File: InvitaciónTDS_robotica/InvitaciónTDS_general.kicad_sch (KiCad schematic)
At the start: 17 parts, among them J1 Voltage Conn, J2 FTDI Connector, Q7 2N2219, SW1 SW_Push, U1 LM358, U2 74LS08

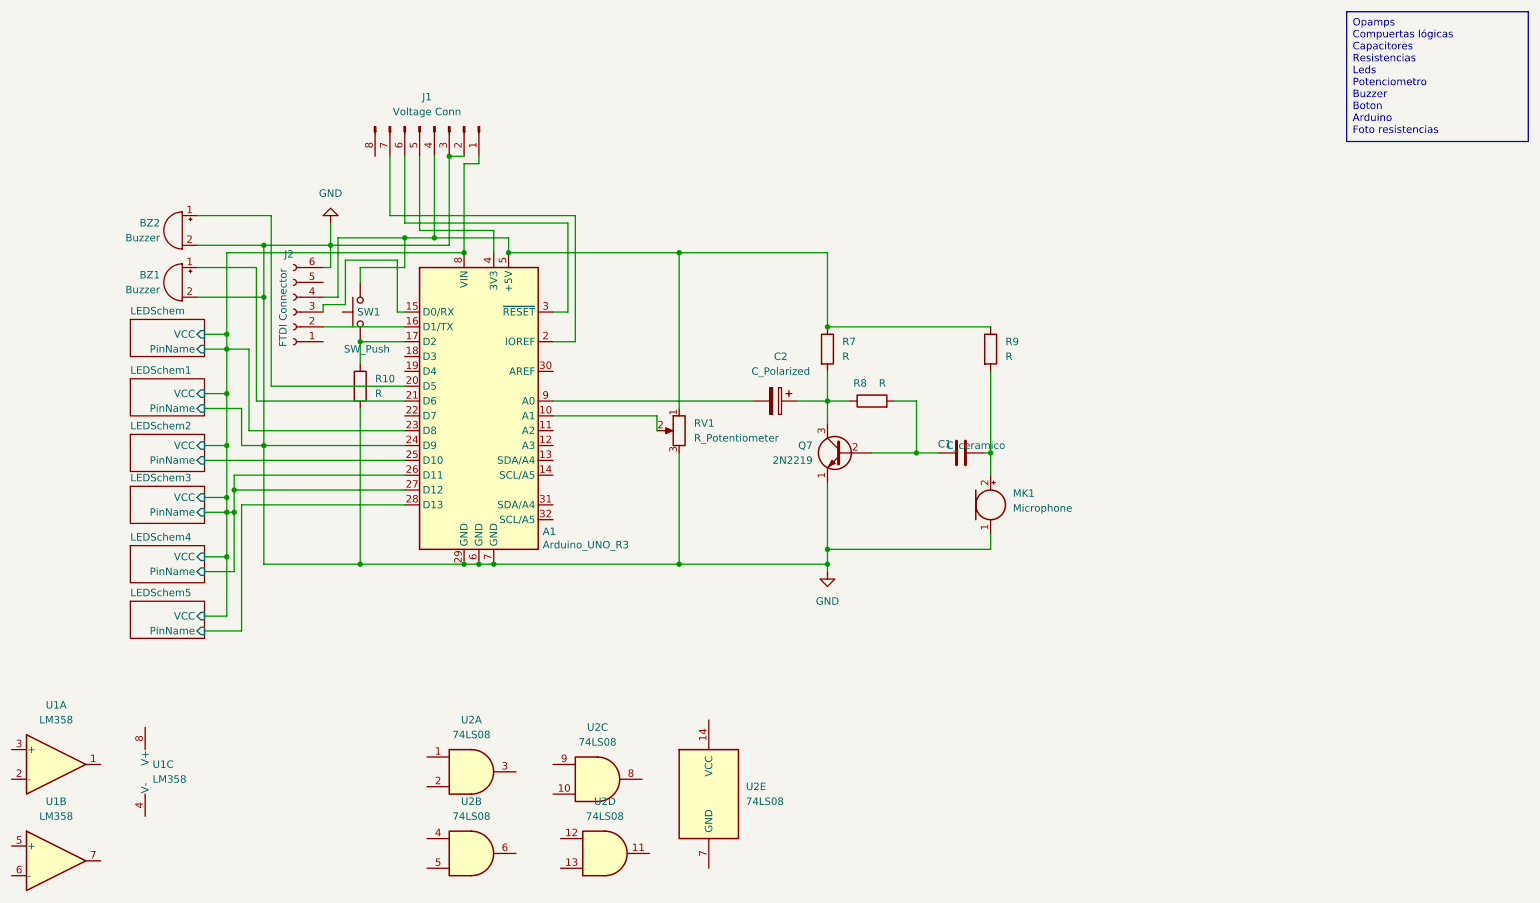
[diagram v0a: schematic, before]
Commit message: update robotica
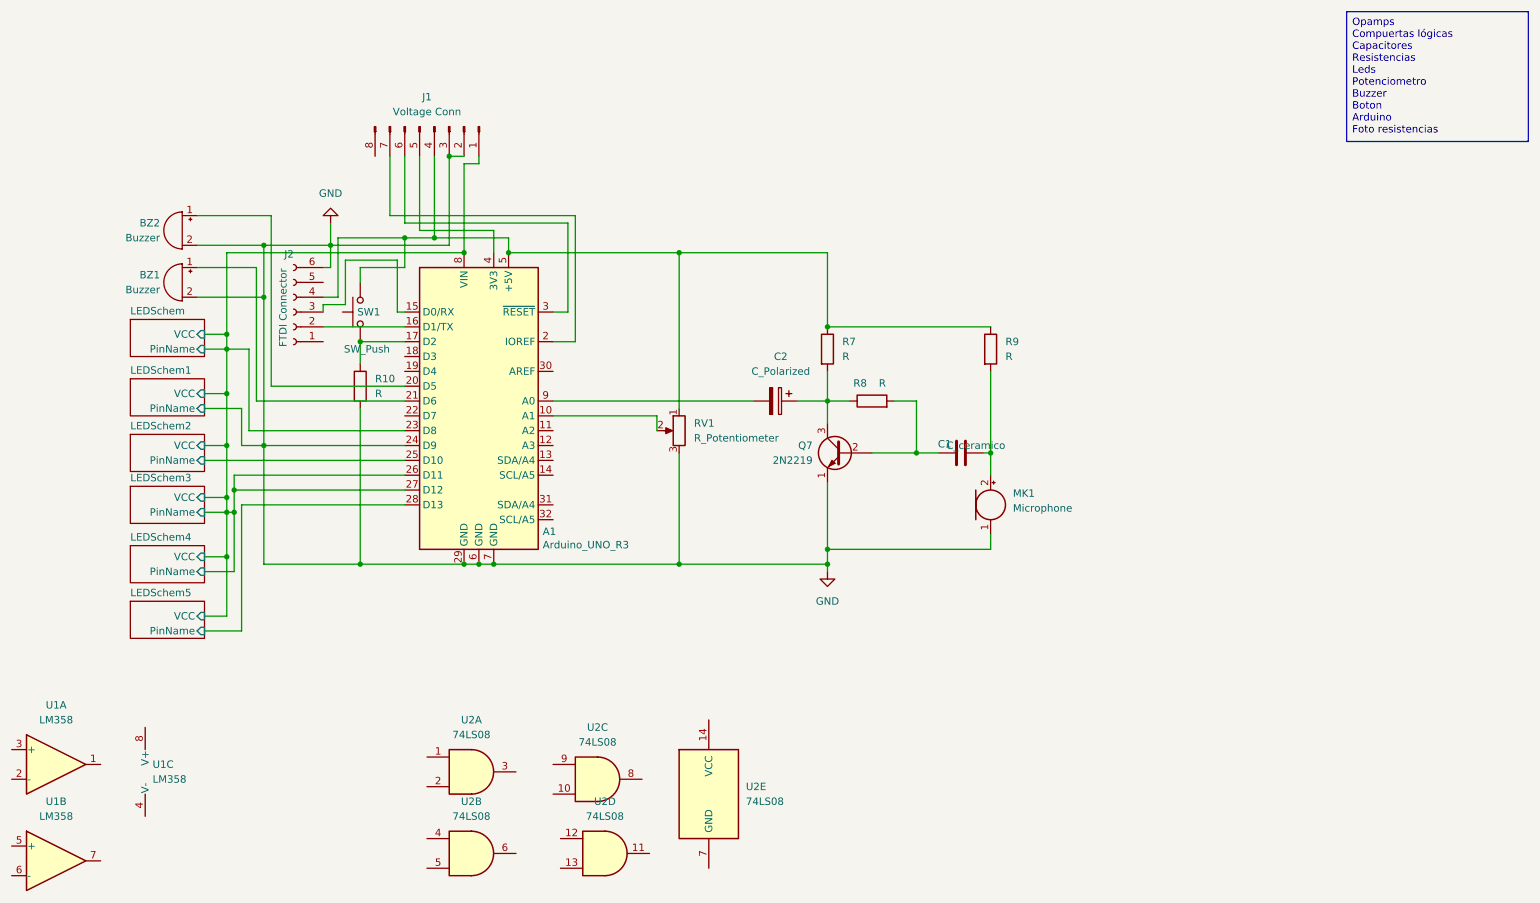
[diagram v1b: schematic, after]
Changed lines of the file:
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@@
 (kicad_sch
-	(version 20231120)
+	(version 20250114)
 	(generator "eeschema")
-	(generator_version "8.0")
+	(generator_version "9.0")
 	(paper "A4")
+	(text_box "Opamps\nCompuertas lógicas\nCapacitores\nResistencias\nLeds\nPotenciometro\nBuzzer\nBoton\nArduino\nFoto resistencias\n"
+		(exclude_from_sim no)
+		(at 251.46 42.545 0)
+		(size 31.115 22.225)
+		(margins 0.9525 0.9525 0.9525 0.9525)
+		(stroke
+			(width 0)
+			(type default)
+		)
+		(fill
+			(type none)
+		)
+		(effects
+			(font
+				(size 1.27 1.27)
+			)
+			(justify left top)
+		)
+	)
 	(junction
 		(at 59.69 128.27)
@@
 			"9QBk43qALbV69VW1GjbMsl2hQiQAAAAAAADc3uxt3QEAAAAAAACUfIRIAAAAAAAAsESIBAAAAAAA"
 			"AEuESAAAAAAAALBEiAQAAAAAAABLhEgAAAAAAACwRIgEAAAAAAAAS4RIAAAAAAAAsESIBAAAAAAA"
-			"AEv/D98C9Ad616Q4AAAAAElFTkSuQmCC"
-		)
-	)
-	(text_box "Opamps\nCompuertas lógicas\nCapacitores\nResistencias\nLeds\nPotenciometro\nBuzzer\nBoton\nArduino\nFoto resistencias\n"
-		(exclude_from_sim no)
-		(at 251.46 42.545 0)
-		(size 31.115 22.225)
-		(stroke
-			(width 0)
-			(type default)
-		)
-		(fill
-			(type none)
-		)
-		(effects
-			(font
-				(size 1.27 1.27)
-			)
-			(justify left top)
+			"AEv/D98C9Ad616Q4AAAAAElFTkSuQmCCAAAAAAAAAAAAAAAAAAAAAAAAAAAAAAAAAAAAAAAAAAAA"
+			"AAAAAAAAAAAAAAAAAAAAAAAAAAAAAAAAAAAAAAAAAAAAAAAAAAAAAAAAAAAAAAAAAAAAAAAAAAAA"
+			"AAAAAAAAAAAAAAAAAAAAAAAAAAAAAAAAAAAAAAAAAAAAAAAAAAAAAAAAAAAAAAAAAAAAAAAAAAAA"
+			"AAAAAAAAAAAAAAAAAAAAAAAAAAAAAAAAAAAAAAAAAAAAAAAAAAAAAAAAAAAAAAAAAAAAAAAAAAAA"
+			"AAAAAAAAAAAAAAAAAAAAAAAAAAAAAAAAAAAAAAAAAAAAAAAAAAAAAAAAAAAAAAAAAAAAAAAAAAAA"
+			"AAAAAAAAAAAAAAAAAAAAAAAAAAAAAAAAAAAAAAAAAAAAAAAAAAAAAAAAAAAAAAAAAAAAAAAAAAAA"
+			"AAAAAAAAAAAAAAAAAAAAAAAAAAAAAAAAAAAAAAAAAAAAAAAAAAAAAAAAAAAAAAAAAAAAAAAAAAAA"
+			"AAAAAAAAAAAAAAAAAAAAAAAAAAAAAAAAAAAAAAAAAAAAAAAAAAAAAAAAAAAAAAAAAAAAAAAAAAAA"
+			"AAAAAAAAAAAAAAAAAAAAAAAAAAAAAAAAAAAAAAAAAAAAAAAAAAAAAAAAAAAAAAAAAAAAAAAAAAAA"
+			"AAAAAAAAAAAAAAAAAAAAAAAAAAAAAAAAAAAAAAAAAAAAAAAAAAAAAAAAAAAAAAAAAAAAAAAAAAAA"
+			"AAAAAAAAAAAAAAAAAAAAAAAAAAAAAAAAAAAAAAAAAAAAAAAAAAAAAAAAAAAAAAAAAAAAAAAAAAAA"
+			"AAAAAAAAAAAAAAAAAAAAAAAAAAAAAAAAAAAAAAAAAAAAAAAAAAAAAAAAAAAAAAAAAAAAAAAAAAAA"
+			"AAAAAAAAAAAAAAAAAAAAAAAAAAAAAAAAAAAAAAAAAAAAAAAAAAAAAAAAAAAAAAAAAAAAAAAAAAAA"
+			"AAAAAAAAAAAAAAAAAAAAAAAAAAAAAAAAAAAAAAAAAAAAAAAAAAAAAAAAAAAAAAAAAAAAAAAAAAAA"
+			"AAAAAAAAAAAAAAAAAAAAAAAAAAAAAAAAAAAAAAAAAAAAAAAAAAAAAAAAAAAAAAAAAAAAAAAAAAAA"
+			"AAAAAAAAAAAAAAAAAAAAAAAAAAAAAAAAAAAAAAAAAAAAAAAAAAAAAAAAAAAAAAAAAAAAAAAAAAAA"
+			"AAAAAAAAAAAAAAAAAAAAAAAAAAAAAAAAAAAAAAAAAAAAAAAAAAAAAAAAAAAAAAAAAAAAAAAAAAAA"
+			"AAAAAAAAAAAAAAAAAAAAAAAAAAAAAAAAAAAAAAAAAAAAAAAAAAAAAAAAAAAAAAAAAAAAAAAAAAAA"
+			"AAAAAAAAAAAAAAAAAAAAAAAAAAAAAA=="
 		)
 	)
@@
 		(at 43.18 95.25)
 		(size 12.7 6.35)
+		(exclude_from_sim no)
+		(in_bom yes)
+		(on_board yes)
+		(dnp no)
 		(stroke
 			(width 0.1524)
@@
 		(at 43.18 123.825)
 		(size 12.7 6.35)
+		(exclude_from_sim no)
+		(in_bom yes)
+		(on_board yes)
+		(dnp no)
 		(stroke
 			(width 0.1524)
@@
 		(at 43.18 143.51)
 		(size 12.7 6.35)
+		(exclude_from_sim no)
+		(in_bom yes)
+		(on_board yes)
+		(dnp no)
 		(stroke
 			(width 0.1524)
@@
 		(at 43.18 133.985)
 		(size 12.7 6.35)
+		(exclude_from_sim no)
+		(in_bom yes)
+		(on_board yes)
+		(dnp no)
 		(stroke
 			(width 0.1524)
@@
 		(at 43.18 114.935)
 		(size 12.7 6.35)
+		(exclude_from_sim no)
+		(in_bom yes)
+		(on_board yes)
+		(dnp no)
 		(stroke
 			(width 0.1524)
@@
 		(at 43.18 105.41)
 		(size 12.7 6.35)
+		(exclude_from_sim no)
+		(in_bom yes)
+		(on_board yes)
+		(dnp no)
 		(stroke
 			(width 0.1524)
@@
 		)
 	)
+	(embedded_fonts no)
 )

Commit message: terminado
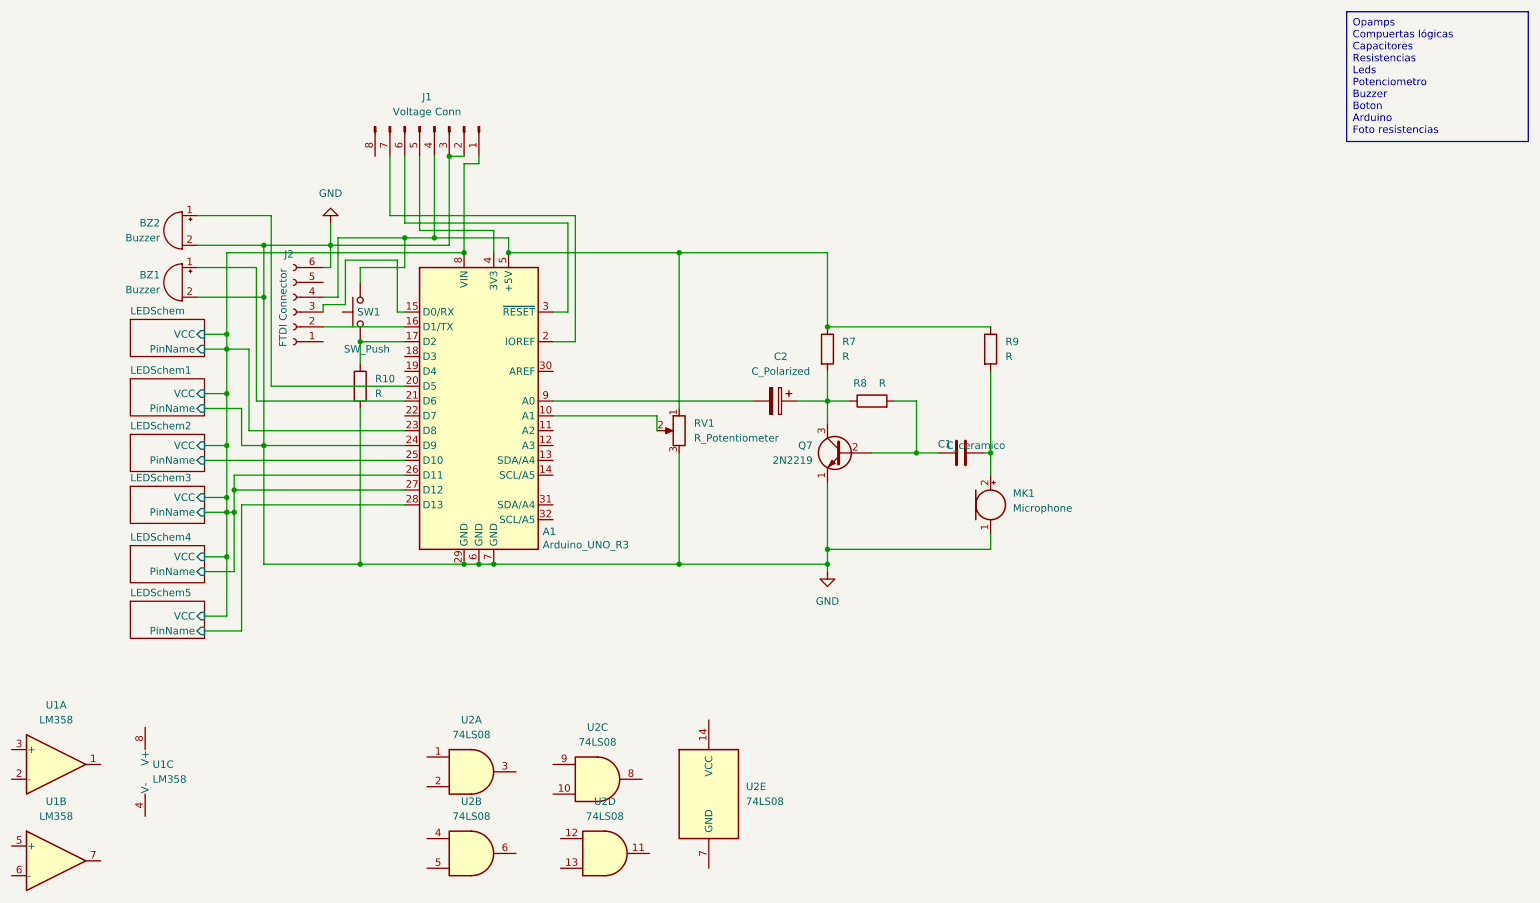
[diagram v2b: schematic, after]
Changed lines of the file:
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@@
 (kicad_sch
-	(version 20250114)
+	(version 20231120)
 	(generator "eeschema")
-	(generator_version "9.0")
+	(generator_version "8.0")
 	(paper "A4")
-	(text_box "Opamps\nCompuertas lógicas\nCapacitores\nResistencias\nLeds\nPotenciometro\nBuzzer\nBoton\nArduino\nFoto resistencias\n"
-		(exclude_from_sim no)
-		(at 251.46 42.545 0)
-		(size 31.115 22.225)
-		(margins 0.9525 0.9525 0.9525 0.9525)
-		(stroke
-			(width 0)
-			(type default)
-		)
-		(fill
-			(type none)
-		)
-		(effects
-			(font
-				(size 1.27 1.27)
-			)
-			(justify left top)
-		)
-	)
 	(junction
 		(at 59.69 128.27)
@@
 			"9QBk43qALbV69VW1GjbMsl2hQiQAAAAAAADc3uxt3QEAAAAAAACUfIRIAAAAAAAAsESIBAAAAAAA"
 			"AEuESAAAAAAAALBEiAQAAAAAAABLhEgAAAAAAACwRIgEAAAAAAAAS4RIAAAAAAAAsESIBAAAAAAA"
-			"AEv/D98C9Ad616Q4AAAAAElFTkSuQmCCAAAAAAAAAAAAAAAAAAAAAAAAAAAAAAAAAAAAAAAAAAAA"
-			"AAAAAAAAAAAAAAAAAAAAAAAAAAAAAAAAAAAAAAAAAAAAAAAAAAAAAAAAAAAAAAAAAAAAAAAAAAAA"
-			"AAAAAAAAAAAAAAAAAAAAAAAAAAAAAAAAAAAAAAAAAAAAAAAAAAAAAAAAAAAAAAAAAAAAAAAAAAAA"
-			"AAAAAAAAAAAAAAAAAAAAAAAAAAAAAAAAAAAAAAAAAAAAAAAAAAAAAAAAAAAAAAAAAAAAAAAAAAAA"
-			"AAAAAAAAAAAAAAAAAAAAAAAAAAAAAAAAAAAAAAAAAAAAAAAAAAAAAAAAAAAAAAAAAAAAAAAAAAAA"
-			"AAAAAAAAAAAAAAAAAAAAAAAAAAAAAAAAAAAAAAAAAAAAAAAAAAAAAAAAAAAAAAAAAAAAAAAAAAAA"
-			"AAAAAAAAAAAAAAAAAAAAAAAAAAAAAAAAAAAAAAAAAAAAAAAAAAAAAAAAAAAAAAAAAAAAAAAAAAAA"
-			"AAAAAAAAAAAAAAAAAAAAAAAAAAAAAAAAAAAAAAAAAAAAAAAAAAAAAAAAAAAAAAAAAAAAAAAAAAAA"
-			"AAAAAAAAAAAAAAAAAAAAAAAAAAAAAAAAAAAAAAAAAAAAAAAAAAAAAAAAAAAAAAAAAAAAAAAAAAAA"
-			"AAAAAAAAAAAAAAAAAAAAAAAAAAAAAAAAAAAAAAAAAAAAAAAAAAAAAAAAAAAAAAAAAAAAAAAAAAAA"
-			"AAAAAAAAAAAAAAAAAAAAAAAAAAAAAAAAAAAAAAAAAAAAAAAAAAAAAAAAAAAAAAAAAAAAAAAAAAAA"
-			"AAAAAAAAAAAAAAAAAAAAAAAAAAAAAAAAAAAAAAAAAAAAAAAAAAAAAAAAAAAAAAAAAAAAAAAAAAAA"
-			"AAAAAAAAAAAAAAAAAAAAAAAAAAAAAAAAAAAAAAAAAAAAAAAAAAAAAAAAAAAAAAAAAAAAAAAAAAAA"
-			"AAAAAAAAAAAAAAAAAAAAAAAAAAAAAAAAAAAAAAAAAAAAAAAAAAAAAAAAAAAAAAAAAAAAAAAAAAAA"
-			"AAAAAAAAAAAAAAAAAAAAAAAAAAAAAAAAAAAAAAAAAAAAAAAAAAAAAAAAAAAAAAAAAAAAAAAAAAAA"
-			"AAAAAAAAAAAAAAAAAAAAAAAAAAAAAAAAAAAAAAAAAAAAAAAAAAAAAAAAAAAAAAAAAAAAAAAAAAAA"
-			"AAAAAAAAAAAAAAAAAAAAAAAAAAAAAAAAAAAAAAAAAAAAAAAAAAAAAAAAAAAAAAAAAAAAAAAAAAAA"
-			"AAAAAAAAAAAAAAAAAAAAAAAAAAAAAAAAAAAAAAAAAAAAAAAAAAAAAAAAAAAAAAAAAAAAAAAAAAAA"
-			"AAAAAAAAAAAAAAAAAAAAAAAAAAAAAA=="
+			"AEv/D98C9Ad616Q4AAAAAElFTkSuQmCC"
+		)
+	)
+	(text_box "Opamps\nCompuertas lógicas\nCapacitores\nResistencias\nLeds\nPotenciometro\nBuzzer\nBoton\nArduino\nFoto resistencias\n"
+		(exclude_from_sim no)
+		(at 251.46 42.545 0)
+		(size 31.115 22.225)
+		(stroke
+			(width 0)
+			(type default)
+		)
+		(fill
+			(type none)
+		)
+		(effects
+			(font
+				(size 1.27 1.27)
+			)
+			(justify left top)
 		)
 	)
@@
 		(at 43.18 95.25)
 		(size 12.7 6.35)
-		(exclude_from_sim no)
-		(in_bom yes)
-		(on_board yes)
-		(dnp no)
 		(stroke
 			(width 0.1524)
@@
 		(at 43.18 123.825)
 		(size 12.7 6.35)
-		(exclude_from_sim no)
-		(in_bom yes)
-		(on_board yes)
-		(dnp no)
 		(stroke
 			(width 0.1524)
@@
 		(at 43.18 143.51)
 		(size 12.7 6.35)
-		(exclude_from_sim no)
-		(in_bom yes)
-		(on_board yes)
-		(dnp no)
 		(stroke
 			(width 0.1524)
@@
 		(at 43.18 133.985)
 		(size 12.7 6.35)
-		(exclude_from_sim no)
-		(in_bom yes)
-		(on_board yes)
-		(dnp no)
 		(stroke
 			(width 0.1524)
@@
 		(at 43.18 114.935)
 		(size 12.7 6.35)
-		(exclude_from_sim no)
-		(in_bom yes)
-		(on_board yes)
-		(dnp no)
 		(stroke
 			(width 0.1524)
@@
 		(at 43.18 105.41)
 		(size 12.7 6.35)
-		(exclude_from_sim no)
-		(in_bom yes)
-		(on_board yes)
-		(dnp no)
 		(stroke
 			(width 0.1524)
@@
 		)
 	)
-	(embedded_fonts no)
 )
